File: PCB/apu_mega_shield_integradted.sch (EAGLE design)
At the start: 78 parts, among them IC1 74AHC573, IC10 DAC, IC11 IS62C1024AL, IC2 4050D, IC3 DS1307, IC4 LP298XS, IC5 S-SMP, IC6 S-DSP, IC7 LM2904, IC8 5x832 SRAM, IC9 5x832 SRAM, Q1 32.768, X1 MICROSDMOLEX, X2 24.576Mhz

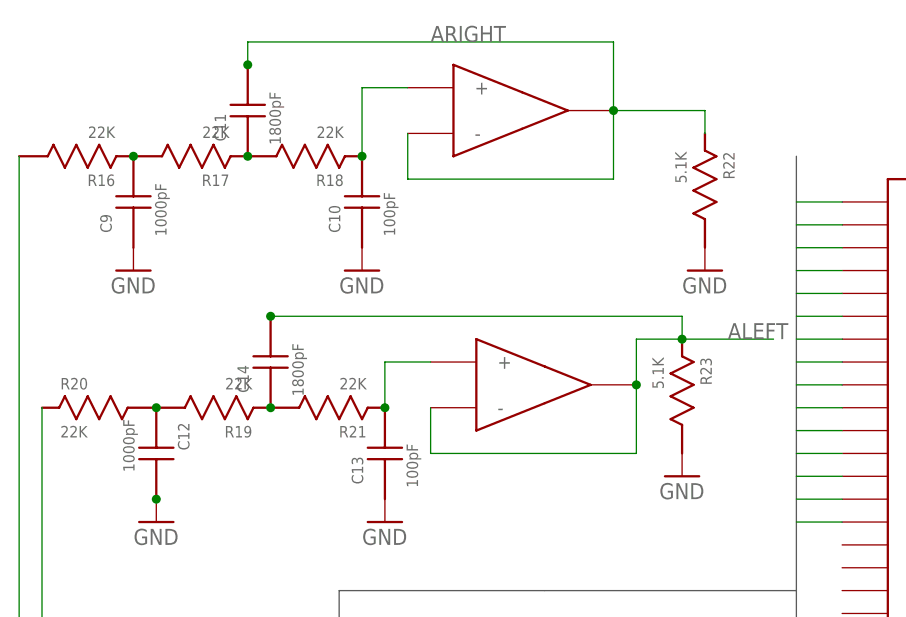
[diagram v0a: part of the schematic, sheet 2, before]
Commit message: Final revisions to the PCB design, hopefully. :)
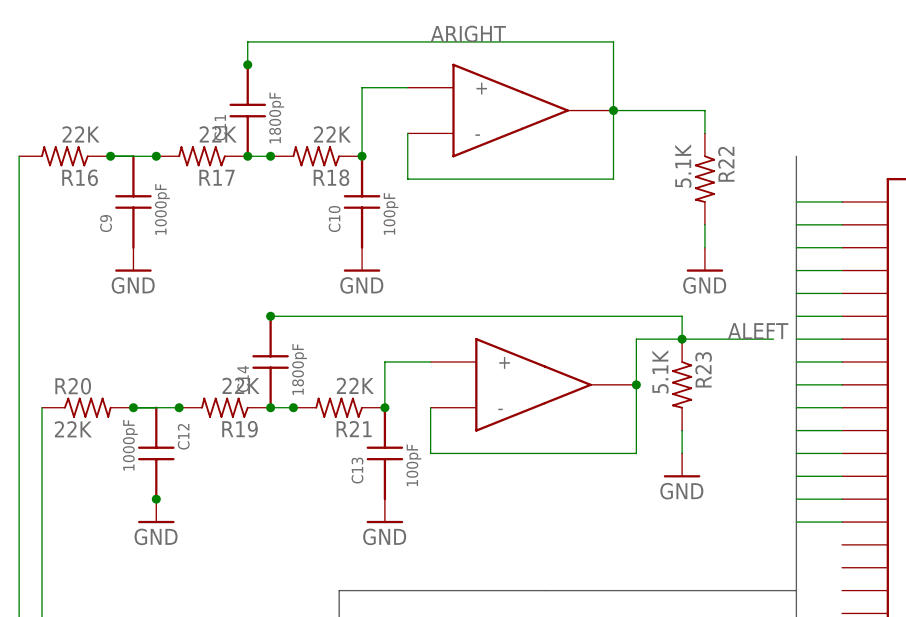
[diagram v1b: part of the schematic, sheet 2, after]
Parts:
- C1, C2, C24, C7: device rcl:C-EUC0805 -> apu_pcb:C0805
- C3, C4, C5, C6: device resistor:C-EUC0805 -> apu_pcb:C0805
- R10, R11, R12, R13, R14, R15, R2, R3, R4, R5, R7, R8, R9: device resistor:R-US_R0805 -> adafruit:R-US_R0805
- R16, R17, R18, R19, R20, R21, R22, R23: device apu_pcb:R0805 -> adafruit:R-US_R0805
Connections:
- net N$14 renamed PWM
- net ALEFT: now also C14.2, R23.1; no longer C14.P$2, R23.P$1
- net ARIGHT: now also C11.2, R22.1; no longer C11.P$2, R22.P$1
- net GND: now also C10.1, C12.2, C13.1, C15.2, C16.2, C17.2, C18.2, C19.2, C20.1, C21.1, C22.1, C23.2, C9.1, R22.2, R23.2, U$4.P$4, U$5.P$4; no longer C10.P$1, C12.P$2, C13.P$1, C15.P$2, C16.P$2, C17.P$2, C18.P$2, C19.P$2, C20.P$1, C21.P$1, C22.P$1, C23.P$2, C9.P$1, R22.P$2, R23.P$2, U$4.PGND1, U$5.PGND1
- net L.OUT: now also R16.2; no longer R16.P$2
- net L1: now also C12.1, R19.2, R20.2; no longer C12.P$1, R19.P$2, R20.P$2
- net L2: now also C14.1, R19.1, R21.2; no longer C14.P$1, R19.P$1, R21.P$2
- net L3: now also C13.2, R21.1; no longer C13.P$2, R21.P$1
- net N$2: now also U$4.P$1; no longer U$4.PSIG
- net N$3: now also U$5.P$1; no longer U$5.PSIG
- net R.OUT: now also R20.1; no longer R20.P$1
- net R1: now also C9.2, R16.1, R17.2; no longer C9.P$2, R16.P$1, R17.P$2
- net R2: now also C11.1, R17.1, R18.2; no longer C11.P$1, R17.P$1, R18.P$2
- net R3: now also C10.2, R18.1; no longer C10.P$2, R18.P$1
- net VCC: now also C15.1, C16.1, C17.1, C18.1, C19.1, C22.2, C23.1; no longer C15.P$1, C16.P$1, C17.P$1, C18.P$1, C19.P$1, C22.P$2, C23.P$1
- net XTAL1: now also C21.2; no longer C21.P$2
- net XTAL2: now also C20.2; no longer C20.P$2
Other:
- moved on the sheet: C1, C2, C24, C3, C4, C5, C6, C7
